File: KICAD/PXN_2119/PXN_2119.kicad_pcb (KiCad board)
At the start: 2 copper layers, 133.5 x 35.2 mm, 94 parts, among them P1 HDR-IDC-2.54-2X3P, P2 SWD, SW1 TS-1187A-B-A-B, U2 SN74HC165N, U3 Micro USB-B 5P_C40942, U4 SN74HC165N, U5 SN74HC165N, U6 SN74HC165N, U7 STM32F103C8T6, U8 AMS1117-3.3, X2 8MHz, X3 32.768kHz

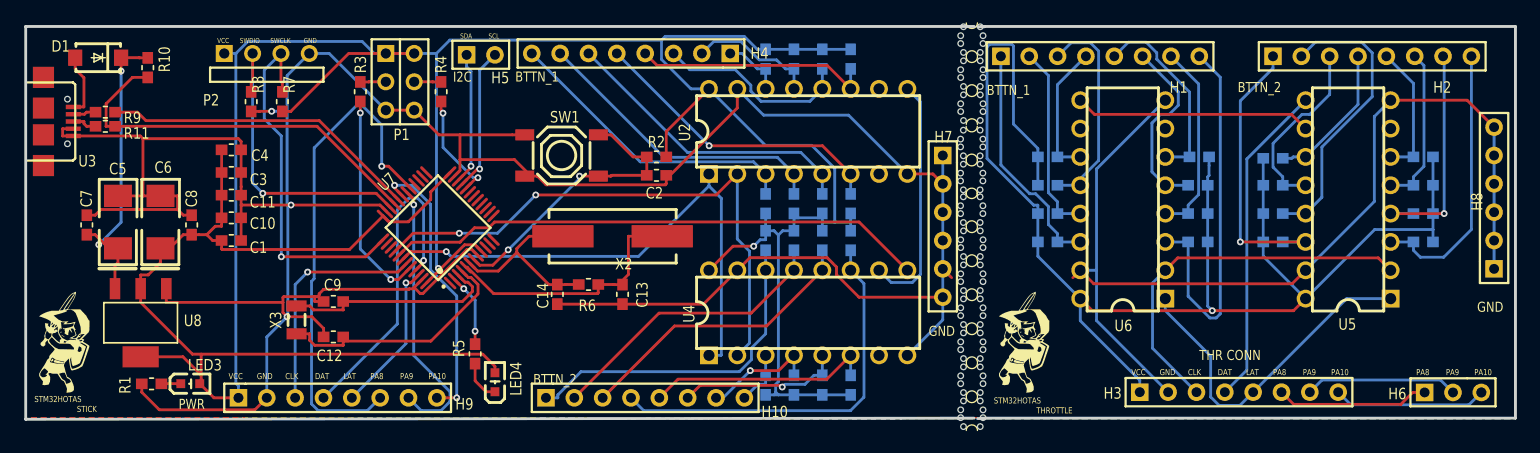
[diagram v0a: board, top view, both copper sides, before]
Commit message: Fixing Routing
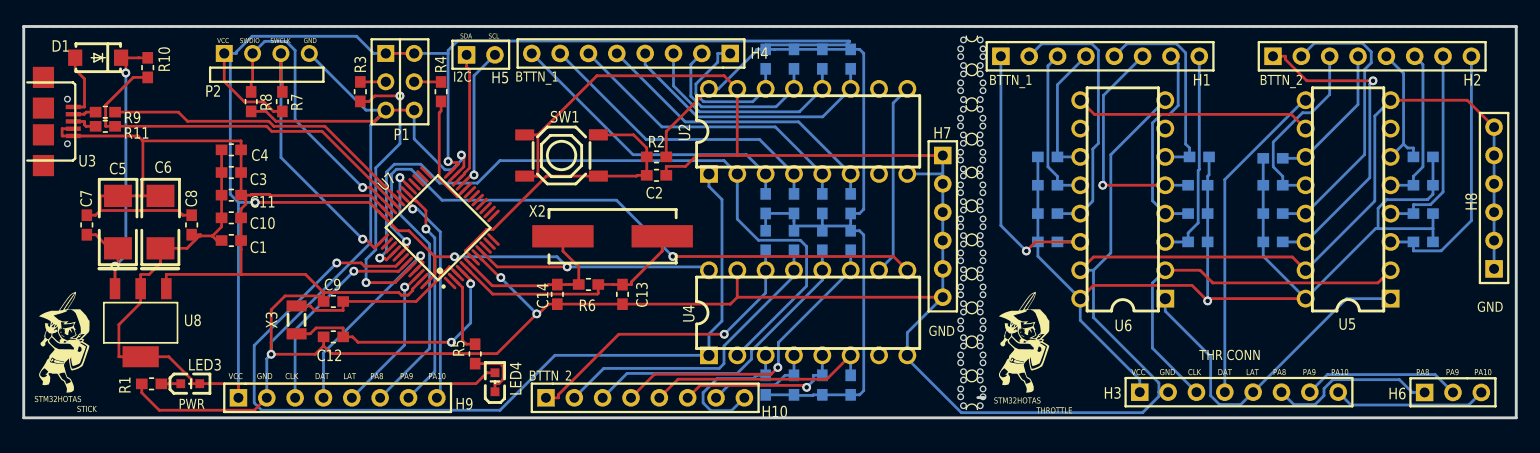
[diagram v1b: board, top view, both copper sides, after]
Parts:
- removed mouse-bite-1mm-slot: VAL**, footprints:mouse-bite-1mm-slot
- added G***: LOGO, LOGO, B.Cu at (104.7, 97.9)
- moved mouse-bite-1mm-slot-1 1.87 mm to (162.7, 113.5)
- moved mouse-bite-1mm-slot-10 1.87 mm to (162.7, 86.1)
- moved mouse-bite-1mm-slot-2 1.87 mm to (162.7, 110.5)
- moved mouse-bite-1mm-slot-11 1.87 mm to (162.7, 83.0)
- moved mouse-bite-1mm-slot-3 1.87 mm to (162.7, 107.4)
- moved mouse-bite-1mm-slot-4 1.87 mm to (162.7, 104.4)
- moved mouse-bite-1mm-slot-5 1.87 mm to (162.7, 101.3)
- moved mouse-bite-1mm-slot-6 1.87 mm to (162.7, 98.3)
- moved mouse-bite-1mm-slot-7 1.87 mm to (162.7, 95.2)
- moved mouse-bite-1mm-slot-8 1.87 mm to (162.7, 92.3)
- moved mouse-bite-1mm-slot-9 1.87 mm to (162.7, 89.2)
- renumbered mouse-bite-1mm-slot to mouse-bite-1mm-slot-1, mouse-bite-1mm-slot to mouse-bite-1mm-slot-10, mouse-bite-1mm-slot to mouse-bite-1mm-slot-11, mouse-bite-1mm-slot to mouse-bite-1mm-slot-2, mouse-bite-1mm-slot to mouse-bite-1mm-slot-3, mouse-bite-1mm-slot to mouse-bite-1mm-slot-4, mouse-bite-1mm-slot to mouse-bite-1mm-slot-5, mouse-bite-1mm-slot to mouse-bite-1mm-slot-6, mouse-bite-1mm-slot to mouse-bite-1mm-slot-7, mouse-bite-1mm-slot to mouse-bite-1mm-slot-8, mouse-bite-1mm-slot to mouse-bite-1mm-slot-9
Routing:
- net GND: track 385.4 -> 455.8 mm, vias 3 -> 4
- net PB6: track 48.3 -> 82.2 mm
- net /VCC_THR: track 123.6 -> 100.5 mm
- net PA8: track 45.4 -> 24.0 mm
- net PB4: track 50.7 -> 67.1 mm, vias 2 -> 1
- net VCC: track 297.6 -> 313.6 mm, vias 2 -> 4
- net Net-(H1-Pad8): track 34.6 -> 19.1 mm
- net PB8: track 28.9 -> 18.1 mm
- net PB5: track 48.6 -> 58.3 mm, vias 0 -> 2
- net Net-(H4-Pad1): track 5.56 -> 14.4 mm
- net Net-(H10-Pad8): track 5.00 -> 13.4 mm
- net Net-(H10-Pad4): track 35.5 -> 27.5 mm, vias 0 -> 1
- net SWCLK: track 32.7 -> 25.6 mm
- net Net-(H1-Pad2): track 17.2 -> 24.3 mm
- net BOOT0: track 19.3 -> 26.3 mm
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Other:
- board size 133.5 x 35.2 mm -> 133.8 x 35.1 mm
